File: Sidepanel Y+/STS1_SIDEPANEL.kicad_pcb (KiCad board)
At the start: 2 copper layers, 82.8 x 100 mm, 49 parts, among them IC1 TMP112AQDRLRQ1, J1 Conn_02x04_Odd_Even, J2 Conn_02x02_Odd_Even, U1 GUVA-C32SM

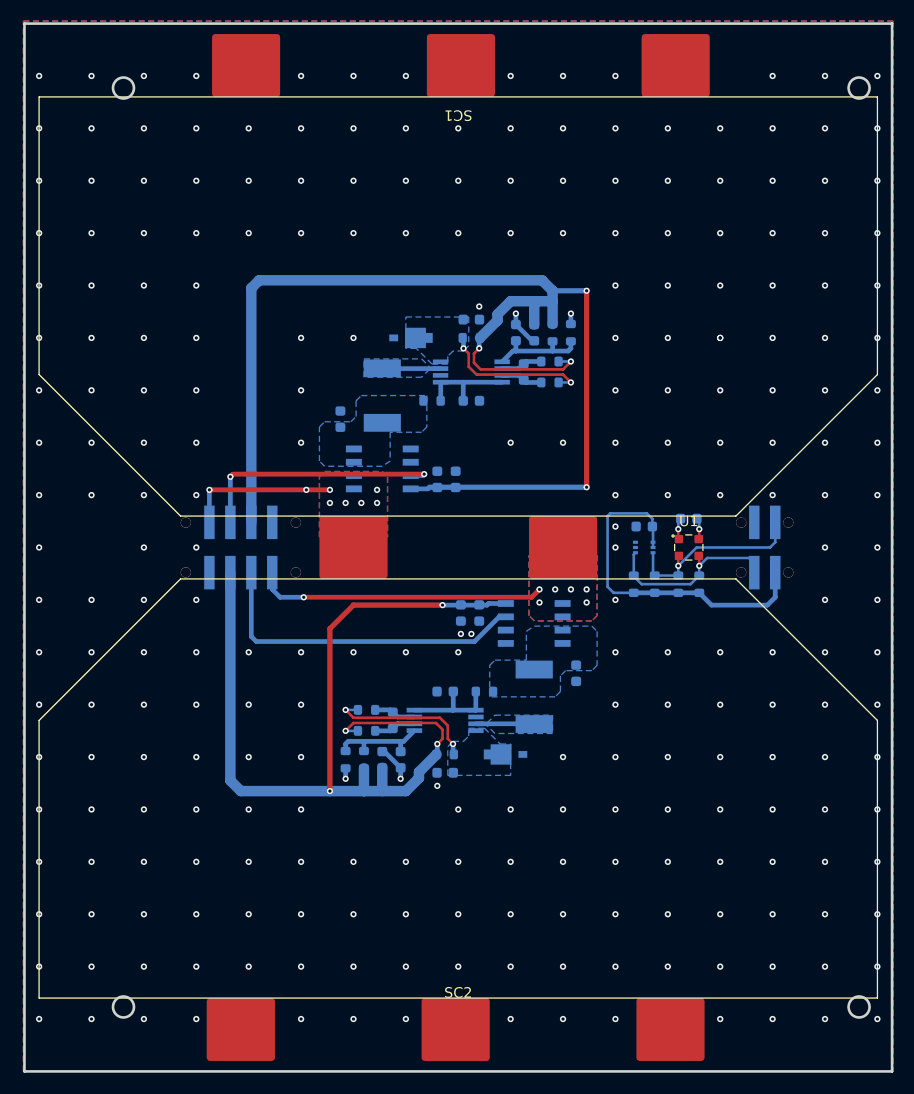
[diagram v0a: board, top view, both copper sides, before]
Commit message: Review Ready for V2.0
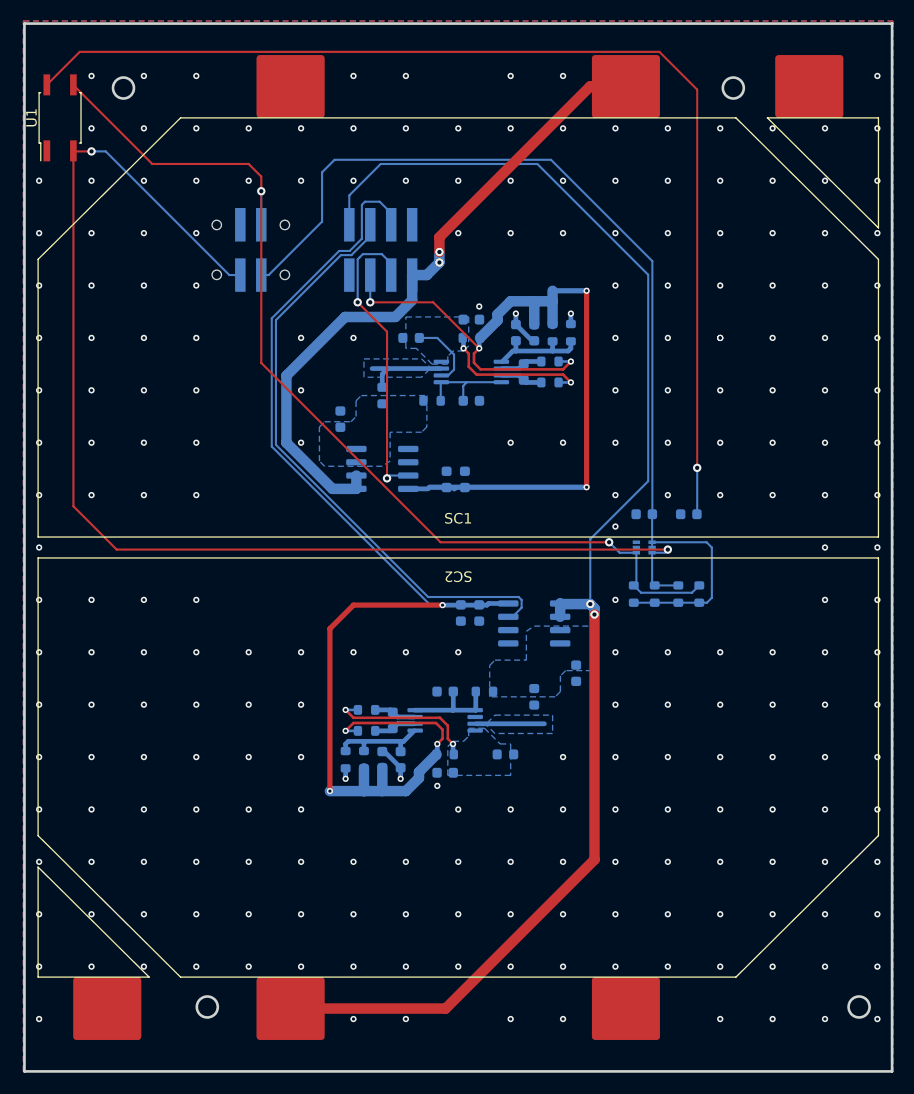
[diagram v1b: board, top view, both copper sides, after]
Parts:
- CUR1, CUR2: footprint SamacSys:SOIC127P600X175-8N -> Package_SO:SOIC-8_3.9x4.9mm_P1.27mm
- DOUT1, DOUT2: footprint SamacSys:STMITE -> Diode_SMD:D_0603_1608Metric
- IC1: footprint SamacSys:SOTFL50P160X60-6N -> Package_TO_SOT_SMD:SOT-563
- J1: footprint SamacSys:M808280842 -> STS_Connector:M808280842
- J2: footprint USER_Passiv:M80-8280442 -> STS_Connector:M808280442
- L_IN1, L_IN2: footprint SamacSys:INDPM5650X530N -> Inductor_SMD:L_0603_1608Metric
- MPPT1, MPPT2: footprint SamacSys:SOP65P640X120-8N -> Package_SO:TSSOP-8_4.4x3mm_P0.65mm
- SC1, SC2: footprint USER_Activ:3G30A_40x80 -> STS_Connector:3G30A_40x80
- U1: footprint USER_Optic:OLGA 2mm x 2,3mm -> Package_SO:SO-4_4.4x3.6mm_P2.54mm
- moved U1 72.7 mm to (87.0, 48.5), turned to 90 degrees
- moved J2 56.7 mm to (105.2, 61.1)
- moved J1 31.4 mm to (117.6, 61.1), turned to 180 degrees
- moved SC1 2.00 mm to (125.0, 68.5), turned to 0 degrees
- moved SC2 2.00 mm to (125.0, 110.5), turned to 180 degrees
- moved C2 1.17 mm to (142.8, 86.3)
- moved RIC1 0.94 mm to (141.8, 93.9)
- moved RIC2 0.94 mm to (143.8, 93.9)
- moved RU1 0.94 mm to (148.0, 93.9)
- moved RU2 0.94 mm to (146.0, 93.9)
- moved C_CUR11 0.89 mm to (123.9, 83.0)
- moved C_CUR21 0.89 mm to (125.6, 83.0)
- moved C1 0.42 mm to (147.0, 86.3)
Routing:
- net /SC2_V+: track 27.7 -> 134.3 mm, vias 7 -> 2
- net /Sensors/VBAT: track 2.06 -> 105.4 mm
- net /SDA: track 18.5 -> 120.3 mm, vias 1 -> 2
- net /SCL: track 17.8 -> 95.9 mm, vias 1 -> 2
- net /+3V3: track 33.2 -> 94.3 mm
- net /SC1_V+: track 14.6 -> 62.8 mm, vias 8 -> 2
- net /MPPT1: track 118.6 -> 81.6 mm, vias 4 -> 5
- net /SC2_I+: track 31.6 -> 57.3 mm
- net /MPPT2: track 93.2 -> 117.7 mm
- net /SC1_I+: track 24.3 -> 29.1 mm
- net GND: track 10.9 -> 15.7 mm, vias 264 -> 243
- net /SolarMPPT/MPPT1_IN: track 6.57 -> 8.58 mm
- removed copper zone on B.Cu, net /SC1_V+
- removed copper zone on F.Cu, net /SC1_V+
- removed copper zone on B.Cu, net /SC2_V+
- removed copper zone on F.Cu, net /SC2_V+
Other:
- outline, holes or cut-outs redrawn
